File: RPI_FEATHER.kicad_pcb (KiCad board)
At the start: 2 copper layers, 63.5 x 53.3 mm, 15 parts, among them J1 FeatherGpIO, J2 Conn_01x12_Female, U1 FeatherFP

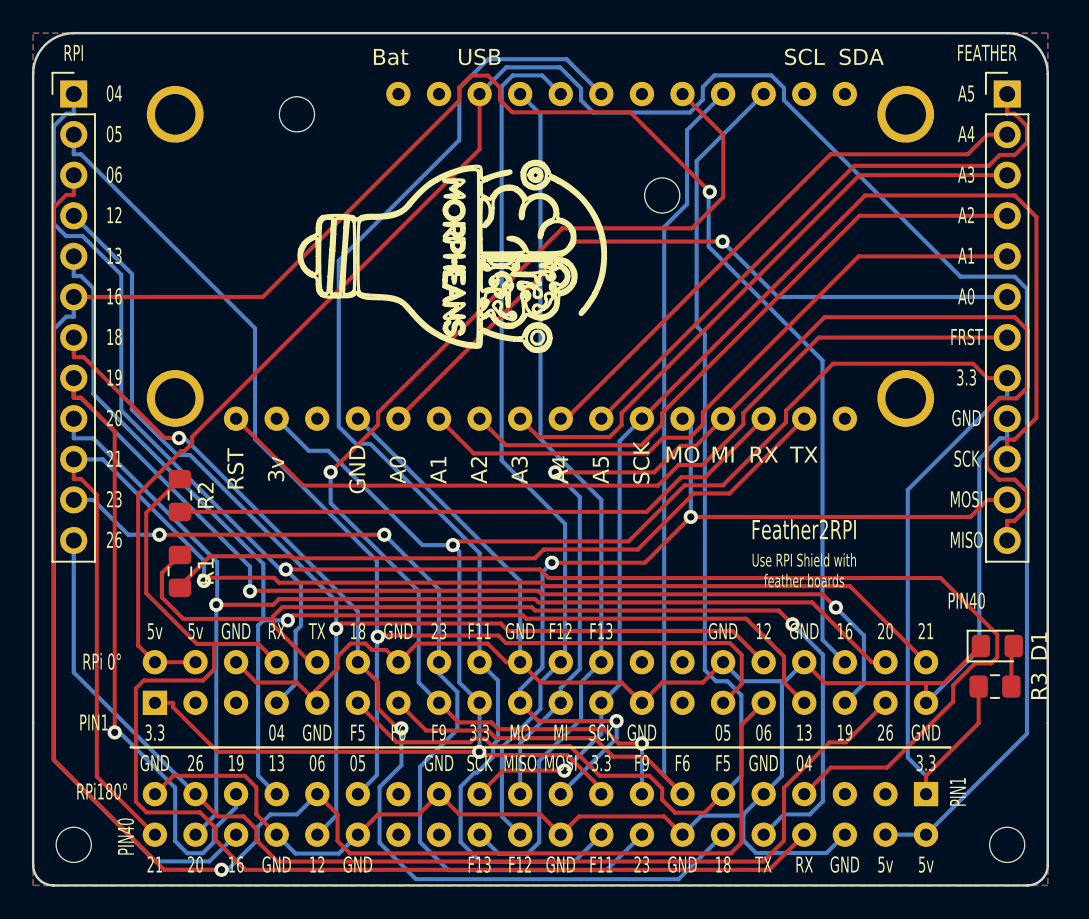
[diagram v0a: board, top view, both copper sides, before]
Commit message: Add files via upload
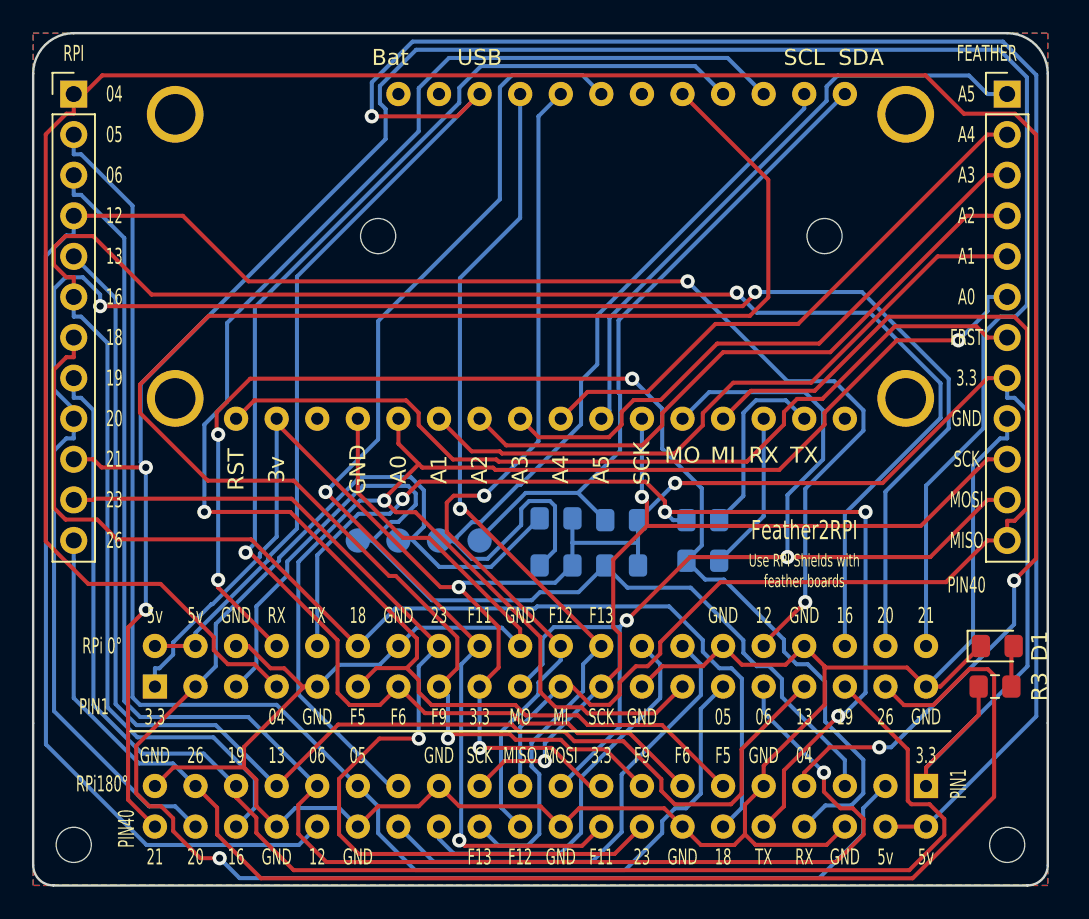
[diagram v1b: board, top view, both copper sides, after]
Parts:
- removed the REF** at (145.9, 57.6)
- removed the REF** at (124.3, 57.6)
- removed REF11, REF22, REF33, REF34: MountingHole_2.2mm_M2, MountingHole:MountingHole_2.2mm_M2
- added H1: MountingHole, MountingHole:MountingHole_2.2mm_M2, F.Cu at (112.8, 94.4)
- added H2: MountingHole, MountingHole:MountingHole_2.2mm_M2, F.Cu at (171.3, 94.4)
- added H3: MountingHole, MountingHole:MountingHole_2.2mm_M2, F.Cu at (131.9, 56.3)
- added H4: MountingHole, MountingHole:MountingHole_2.2mm_M2, F.Cu at (159.8, 56.3)
- added J3: Conn_01x04_Female, 18650:4padsfree, B.Cu at (126.8, 75.4)
- added R4: 4.7k, Resistor_SMD:R_0805_2012Metric_Pad1.15x1.40mm_HandSolder, B.Cu at (143.0, 76.9)
- added R5: 4.7k, Resistor_SMD:R_0805_2012Metric_Pad1.15x1.40mm_HandSolder, B.Cu at (147.1, 76.9)
- added R6: 4.7k, Resistor_SMD:R_0805_2012Metric_Pad1.15x1.40mm_HandSolder, B.Cu at (147.1, 74.1)
- added R7: 4.7k, Resistor_SMD:R_0805_2012Metric_Pad1.15x1.40mm_HandSolder, B.Cu at (143.0, 74.0)
- added REF**: LOGOMORH, 18650:LOGOMORH, B.Cu at (132.8, 56.7)
- R1, R2: moved to B.Cu
- moved R2 33.0 mm to (152.2, 76.6), turned to 0 degrees
- moved R1 32.9 mm to (152.2, 74.1), turned to 0 degrees
- moved PI1 1.02 mm to (117.9, 83.2)
- moved PI2 0.51 mm to (166.2, 92.0)
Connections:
- PI1 pad 26: (no net) -> Net-(PI1-Pad26)
- PI1 pad 27: (no net) -> /A0
- PI1 pad 28: (no net) -> Net-(PI1-Pad28)
- PI1 pad 3: (no net) -> SDA
- PI1 pad 5: (no net) -> SCL
- PI2 pad 26: (no net) -> Net-(PI1-Pad26)
- PI2 pad 27: (no net) -> /A0
- PI2 pad 28: (no net) -> Net-(PI1-Pad28)
- PI2 pad 3: (no net) -> SDA
- PI2 pad 5: (no net) -> SCL
- U1 pad 1: (no net) -> /FSDA
- U1 pad 2: (no net) -> /FSCL
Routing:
- net SDA: track 0.00 -> 97.1 mm, vias 0 -> 1
- net SCL: track 0.00 -> 64.4 mm
- net /A0: track 44.1 -> 99.8 mm, vias 1 -> 2
- net /GPIO21: track 85.4 -> 139.8 mm, vias 1 -> 2
- net /FSCL: track 0.00 -> 51.6 mm
- net /GPIO12: track 74.4 -> 125.9 mm, vias 1 -> 2
- net /GPIO4: track 110.6 -> 159.2 mm, vias 1 -> 2
- net /GPIO20: track 74.7 -> 118.1 mm, vias 1 -> 2
- net /FSDA: track 0.00 -> 41.8 mm
- net Net-(R1-Pad2): track 43.6 -> 12.0 mm
- net /F9: track 73.8 -> 104.6 mm, vias 2 -> 1
- net Net-(PI1-Pad28): track 0.00 -> 29.8 mm
- net Net-(R2-Pad2): track 38.9 -> 10.0 mm
- net /F5: track 74.4 -> 100.9 mm, vias 0 -> 1
- net Net-(PI1-Pad26): track 0.00 -> 24.8 mm
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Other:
- board text added: "FSCL"
- board text added: "FSDA"
- board text added: "RSCL"
- board text added: "RSDA"
- board text added: "Use RPI Shields with feather boards"
- board text removed: "Use RPI Shield with feather boards"
